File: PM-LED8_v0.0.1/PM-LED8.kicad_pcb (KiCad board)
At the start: 2 copper layers, 29.8 x 99.8 mm, 26 parts, among them J1 AFA07-S10FCC-00, J2 AFA07-S10FCC-00, J3 AFA07-S10FCC-00, J4 AFA07-S10FCC-00

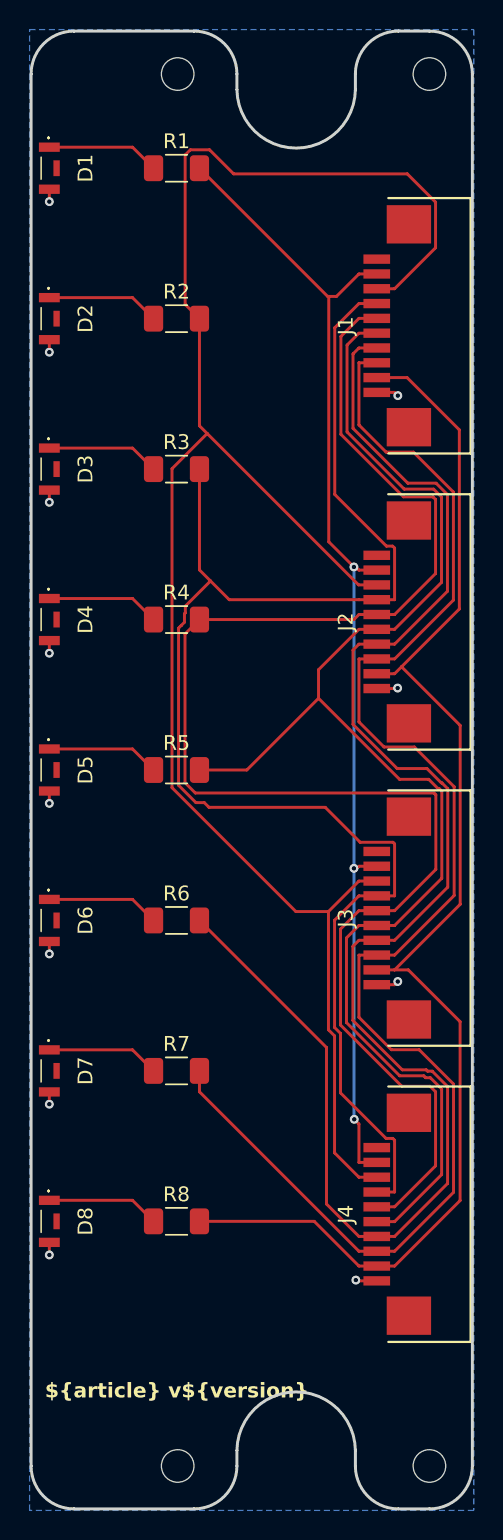
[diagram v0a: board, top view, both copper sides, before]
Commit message: update
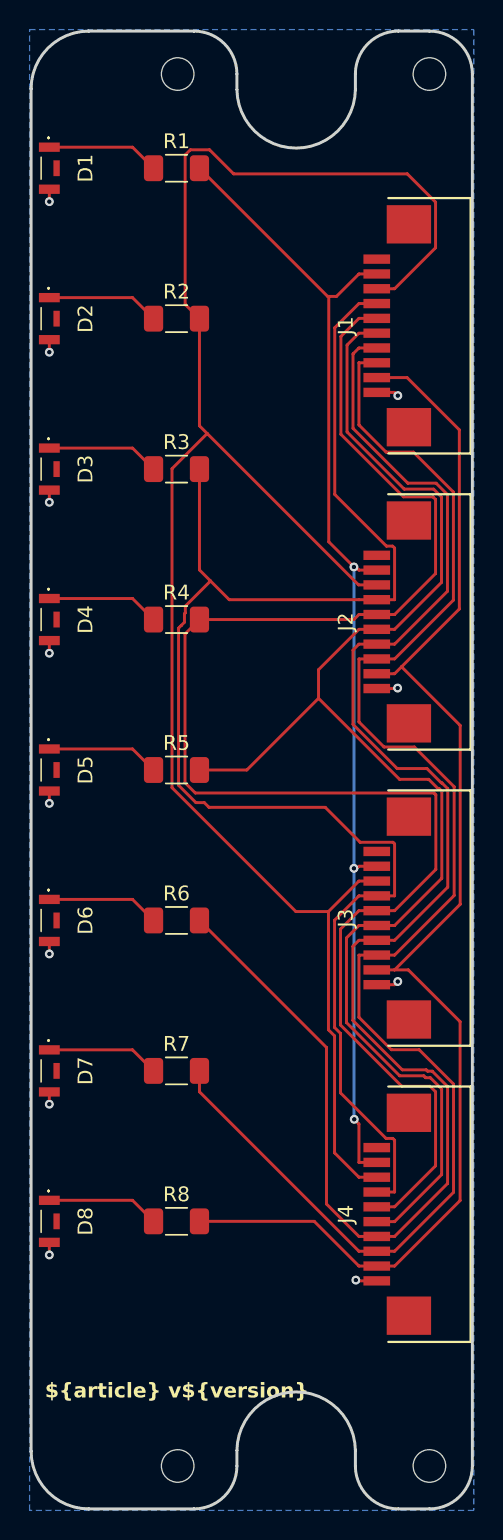
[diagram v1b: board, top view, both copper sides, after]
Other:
- outline, holes or cut-outs redrawn
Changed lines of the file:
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@@
 		(pad_to_mask_clearance 0)
 		(allow_soldermask_bridges_in_footprints no)
-		(grid_origin 60.72 80.48)
+		(aux_axis_origin 65.8 100.8)
+		(grid_origin 65.8 100.8)
 		(pcbplotparams
 			(layerselection 0x00010fc_ffffffff)
@@
 		(layer "Cmts.User")
 	)
+	(gr_arc
+		(start 50.9 54.8)
+		(mid 52.042284 52.042284)
+		(end 54.8 50.9)
+		(stroke
+			(width 0.2)
+			(type default)
+		)
+		(layer "Edge.Cuts")
+	)
 	(gr_line
 		(start 64.8 53.8)
@@
 	(gr_line
 		(start 61.9 150.7)
-		(end 53.8 150.7)
+		(end 54.8 150.7)
 		(stroke
 			(width 0.2)
@@
 	)
 	(gr_line
-		(start 50.9 147.8)
-		(end 50.9 53.8)
+		(start 50.9 146.8)
+		(end 50.9 54.8)
 		(stroke
 			(width 0.2)
@@
 		(layer "Edge.Cuts")
 	)
-	(gr_arc
-		(start 53.8 150.7)
-		(mid 51.74939 149.85061)
-		(end 50.9 147.8)
-		(stroke
-			(width 0.2)
-			(type default)
-		)
-		(layer "Edge.Cuts")
-	)
 	(gr_line
 		(start 80.7 53.8)
@@
 		(layer "Edge.Cuts")
 	)
-	(gr_arc
-		(start 50.9 53.8)
-		(mid 51.74939 51.74939)
-		(end 53.8 50.9)
-		(stroke
-			(width 0.2)
-			(type default)
-		)
-		(layer "Edge.Cuts")
-	)
 	(gr_line
 		(start 72.8 54.85)
@@
 	)
 	(gr_line
-		(start 53.8 50.9)
+		(start 54.8 50.9)
 		(end 61.9 50.9)
 		(stroke
@@
 		(stroke
 			(width 0.2)
+			(type default)
+		)
+		(layer "Edge.Cuts")
+	)
+	(gr_arc
+		(start 54.8 150.7)
+		(mid 52.042284 149.557716)
+		(end 50.9 146.8)
+		(stroke
+			(width 0.2)
